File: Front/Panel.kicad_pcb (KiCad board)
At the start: 2 copper layers, 25 x 200 mm, 11 parts

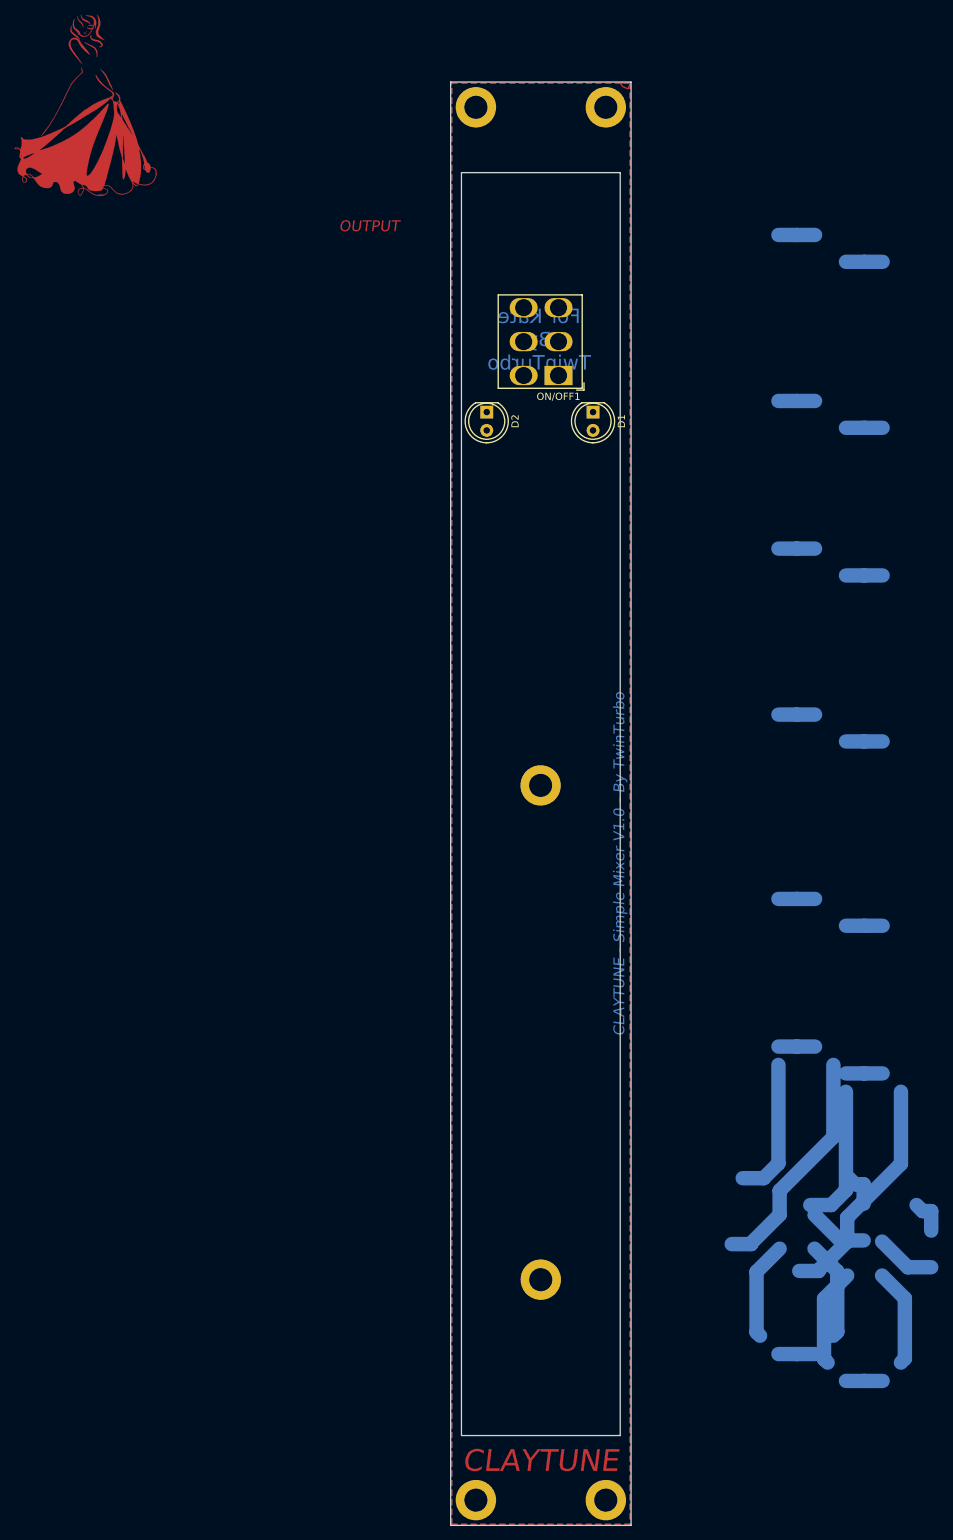
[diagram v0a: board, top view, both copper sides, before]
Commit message: FP Holes Added
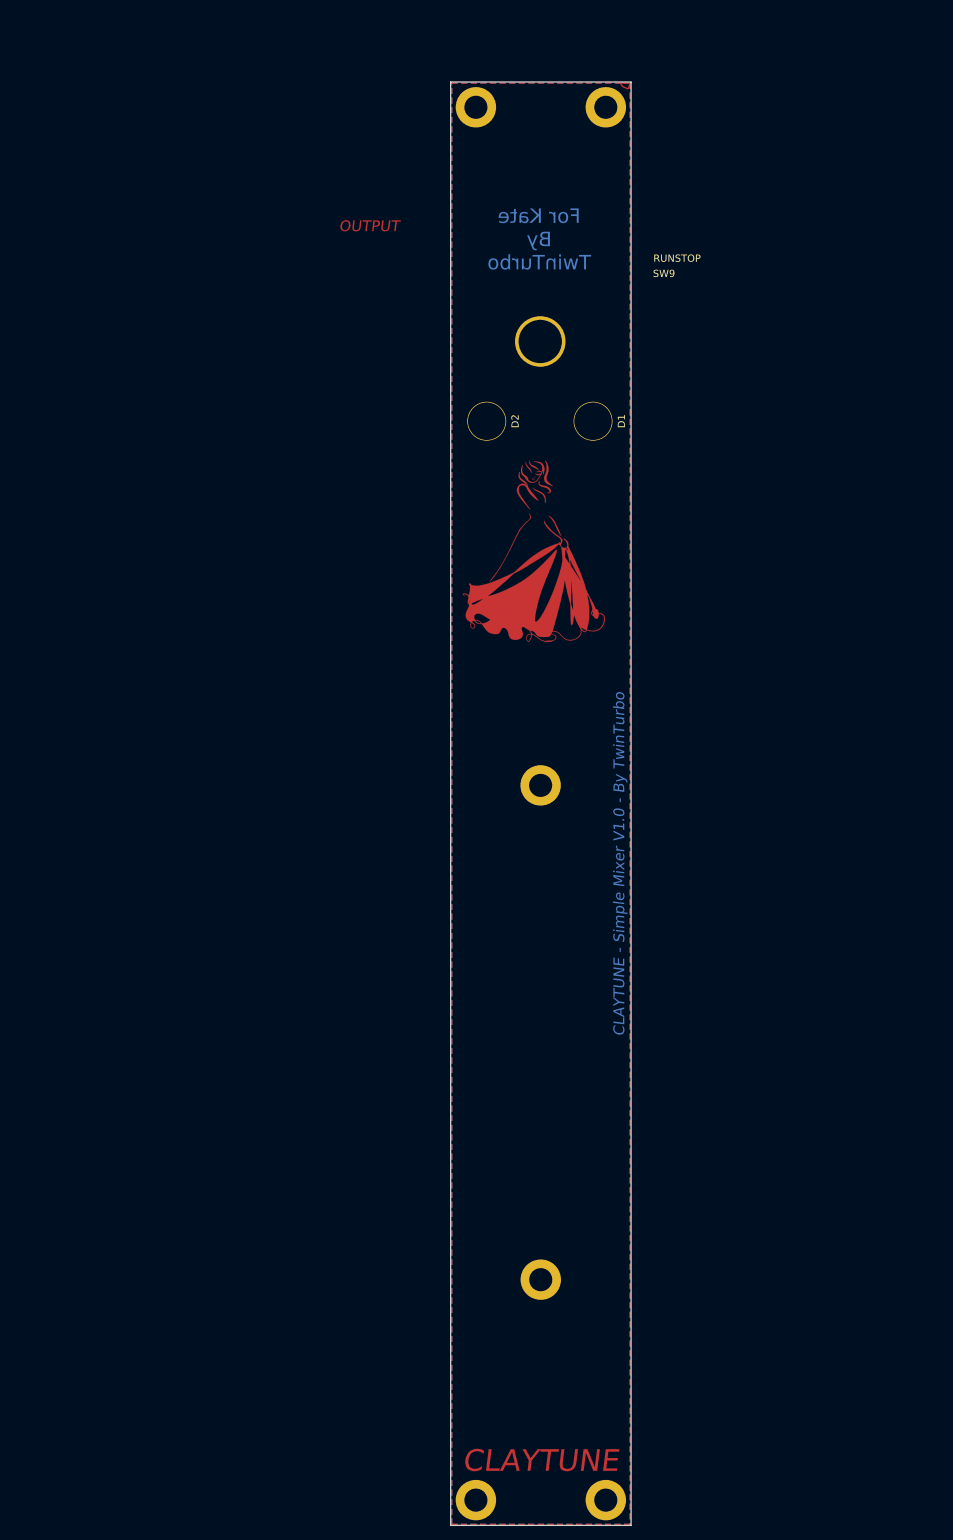
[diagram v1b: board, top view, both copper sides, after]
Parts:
- removed ON/OFF1: SW_DPST, RobsFoots:SW_CK_Lever_DPDT_72xx_CircularHoles
- added SW9: RUNSTOP, RobsFoots:FP-MINITOGLE, F.Cu at (91.7, 54.7)
- D1, D2: footprint LED_THT:LED_D5.0mm -> RobsFoots:FP-LED_D5.0mm
- moved G*** 106.3 mm to (91.5, 131.0)
- moved G*** 87.6 mm to (90.8, 83.2)
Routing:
- net (no net): track 255.6 -> 0.00 mm
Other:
- outline, holes or cut-outs redrawn
